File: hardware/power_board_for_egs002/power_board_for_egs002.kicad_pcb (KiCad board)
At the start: 2 copper layers, 150 x 100 mm, 98 parts, among them J1 +HV, J11 +HV_TO_12, J12 +HV_TO_12, J13 HV_TO_12V, J14 12V_TO_5V, J2 +12V, J21 Conn_01x02, J22 Conn_01x03, J23 Conn_01x02, J24 HV_SENSE_SELECT_A, J25 HV_SENSE_SELECT_B, J26 Conn_01x02, J3 +5V, J4 BRIGDE_OUT_2, J5 BRIGDE_OUT_1, J6 HV_SENSE, Q21 TK40E06N1, Q22 TK40E06N1, Q23 TK40E06N1, Q24 TK40E06N1, Q25 TK40E06N1, Q26 TK40E06N1, Q27 TK40E06N1, Q28 TK40E06N1, U1 EGS002, U2 SK68-100SA

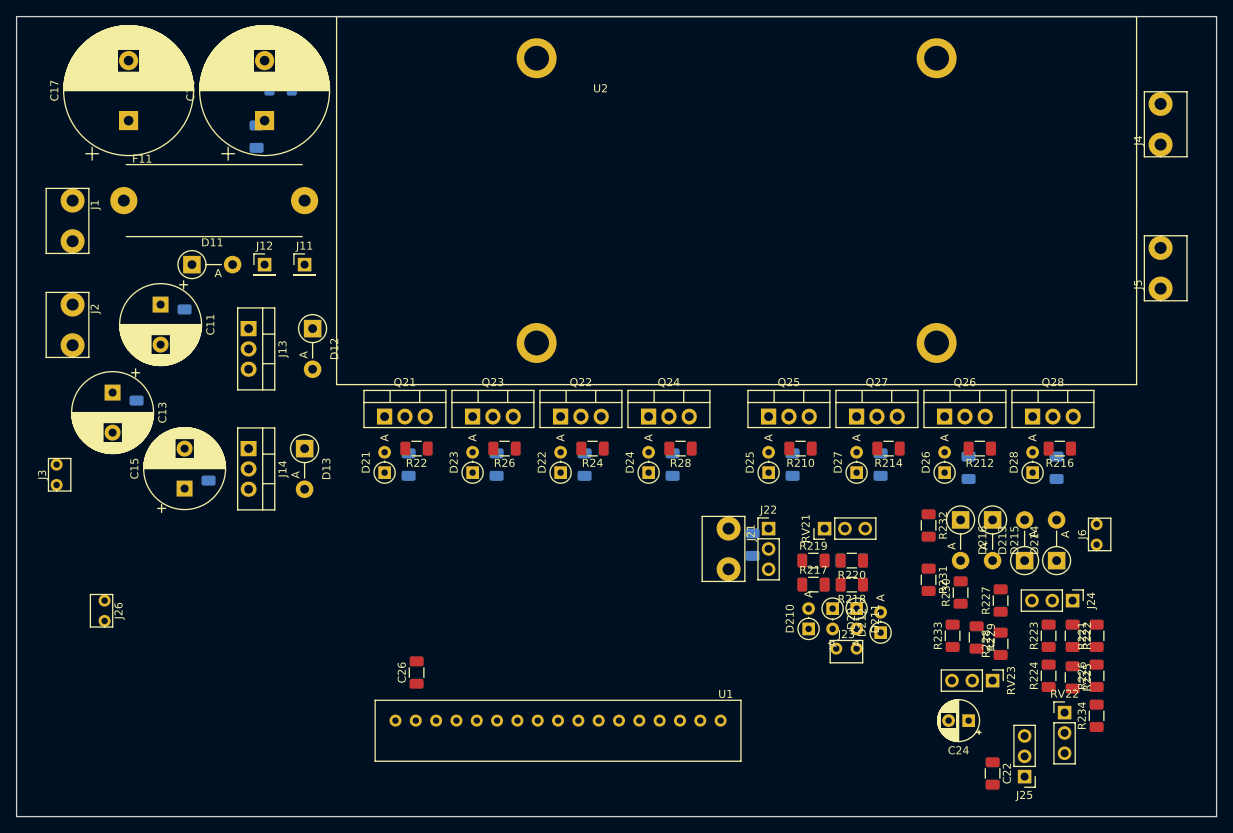
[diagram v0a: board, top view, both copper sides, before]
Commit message: continue pcb work
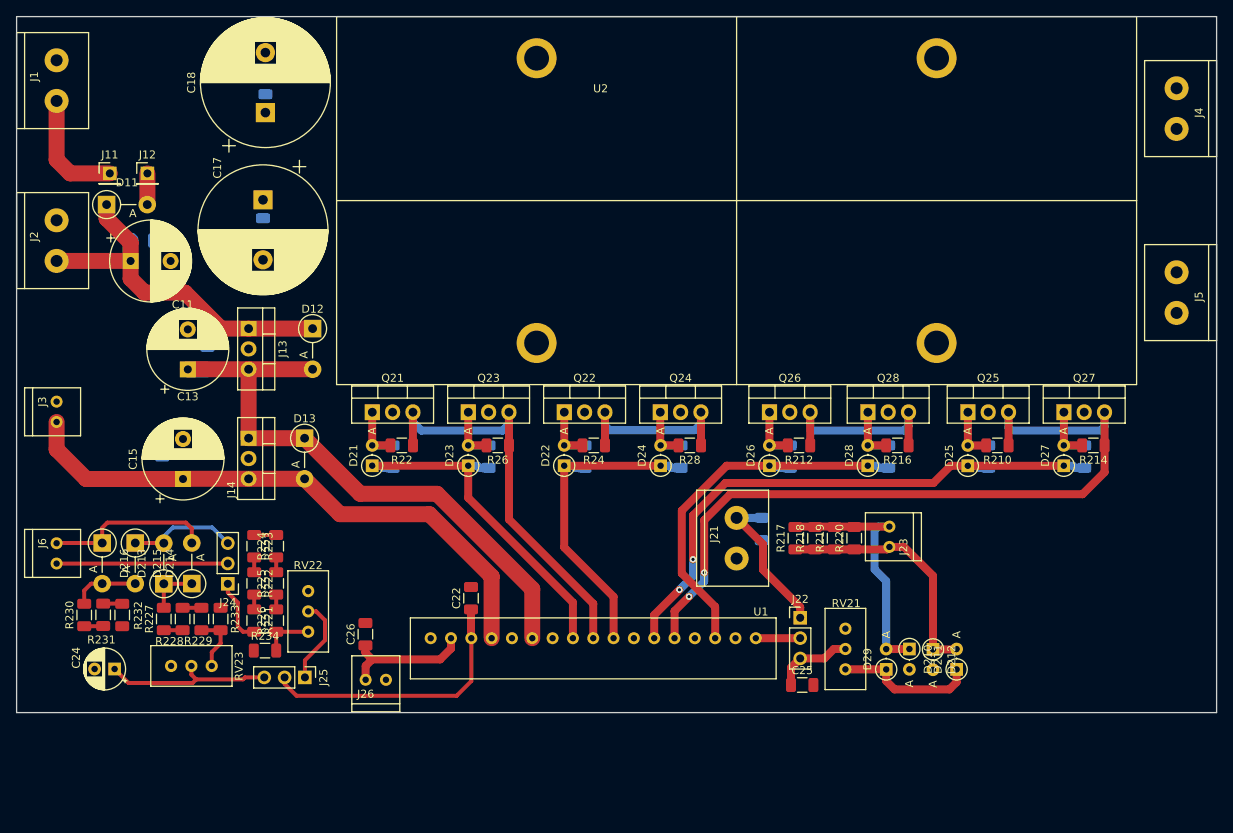
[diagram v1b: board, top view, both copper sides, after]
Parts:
- removed F11: Fuse_Small, power_board_for_egs002:696101000002
- C25: moved to F.Cu
- RV21, RV22, RV23: footprint Connector_PinHeader_2.54mm:PinHeader_1x03_P2.54mm_Vertical -> power_board_for_egs002:r_multiturn
- moved J6 130.0 mm to (40.0, 99.1)
- moved R230 109.6 mm to (43.5, 106.8)
- moved D214 108.1 mm to (56.9, 102.9)
- moved D213 107.6 mm to (53.4, 102.9)
- moved D216 107.3 mm to (45.7, 97.8)
- moved D215 107.2 mm to (49.8, 97.8)
- moved C24 106.9 mm to (47.2, 113.5)
- moved J24 105.6 mm to (61.4, 102.9), turned to 180 degrees
- moved R221 105.3 mm to (64.7, 107.5), turned to 270 degrees
- moved R227 104.6 mm to (53.4, 107.3)
- moved R234 104.3 mm to (66.0, 111.2), turned to 0 degrees
- moved R231 103.3 mm to (45.8, 106.8)
- moved R226 102.8 mm to (67.5, 107.5)
- moved R222 102.5 mm to (64.7, 102.8)
- moved R228 102.3 mm to (55.8, 107.3), turned to 270 degrees
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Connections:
- C110 pad 1: /PowerSupply/+HV_OUT -> /PowerSupply/+HV_IN
- C17 pad 1: /PowerSupply/+HV_OUT -> /PowerSupply/+HV_IN
- C18 pad 1: /PowerSupply/+HV_OUT -> /PowerSupply/+HV_IN
- C19 pad 1: /PowerSupply/+HV_OUT -> /PowerSupply/+HV_IN
- J11 pad 1: /PowerSupply/+HV_OUT -> /PowerSupply/+HV_IN
- J21 pad 1: Net-(J21-Pad1) -> GND
- J21 pad 2: GND -> Net-(J21-Pad2)
- J22 pad 1: Net-(J21-Pad1) -> Net-(J21-Pad2)
- Q21 pad 2: /PowerSupply/+HV_OUT -> /PowerSupply/+HV_IN
- Q22 pad 3: Net-(J21-Pad1) -> Net-(J21-Pad2)
- Q23 pad 2: /PowerSupply/+HV_OUT -> /PowerSupply/+HV_IN
- Q24 pad 3: Net-(J21-Pad1) -> Net-(J21-Pad2)
- Q25 pad 2: /PowerSupply/+HV_OUT -> /PowerSupply/+HV_IN
- Q26 pad 3: Net-(J21-Pad1) -> Net-(J21-Pad2)
- Q27 pad 2: /PowerSupply/+HV_OUT -> /PowerSupply/+HV_IN
- Q28 pad 3: Net-(J21-Pad1) -> Net-(J21-Pad2)
- R212 pad 1: Net-(J21-Pad1) -> Net-(J21-Pad2)
- R216 pad 1: Net-(J21-Pad1) -> Net-(J21-Pad2)
- R217 pad 1: GND -> Net-(D211-Pad2)
- R217 pad 2: Net-(D211-Pad1) -> Net-(D210-Pad1)
- R218 pad 1: GND -> Net-(D211-Pad2)
- R218 pad 2: Net-(D211-Pad1) -> Net-(D210-Pad1)
- R219 pad 1: GND -> Net-(D211-Pad2)
- R219 pad 2: Net-(D211-Pad1) -> Net-(D210-Pad1)
- R220 pad 1: GND -> Net-(D211-Pad2)
- R220 pad 2: Net-(D211-Pad1) -> Net-(D210-Pad1)
- R235 pad 1: Net-(J21-Pad1) -> Net-(J21-Pad2)
- R24 pad 1: Net-(J21-Pad1) -> Net-(J21-Pad2)
- R28 pad 1: Net-(J21-Pad1) -> Net-(J21-Pad2)
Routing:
- net /PowerBoard/1_VS: track 0.00 -> 96.5 mm, vias 0 -> 2
- net /PowerSupply/+12V_OUT: track 0.00 -> 76.1 mm
- net /PowerSupply/+5V_IN: track 0.00 -> 74.7 mm
- net /PowerBoard/1_HO: track 0.00 -> 71.6 mm, vias 0 -> 2
- net Net-(J21-Pad2): track 0.00 -> 67.8 mm
- net /PowerBoard/2_VS: track 0.00 -> 52.3 mm
- net /PowerBoard/1_LO: track 0.00 -> 48.6 mm
- net /PowerSupply/+12V_IN: track 0.00 -> 47.6 mm
- net /PowerBoard/2_HO: track 0.00 -> 44.3 mm
- net /PowerBoard/2_LO: track 0.00 -> 41.4 mm
- net /PowerBoard/V_FB: track 0.00 -> 34.5 mm
- net Net-(D210-Pad1): track 0.00 -> 32.2 mm
- net Net-(D211-Pad2): track 0.00 -> 31.0 mm
- net Net-(C24-Pad1): track 0.00 -> 21.7 mm
- net /PowerBoard/HV_SENSE_L: track 0.00 -> 21.4 mm
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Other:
- board size 150 x 100 mm -> 150 x 87 mm
